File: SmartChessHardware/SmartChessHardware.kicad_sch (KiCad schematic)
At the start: 28 parts, among them IC1 Pi-Zero-UART, IC2 Arduino_UNO_R3, IC3 MCP23017x-x-SO, J1 Barrel_Jack

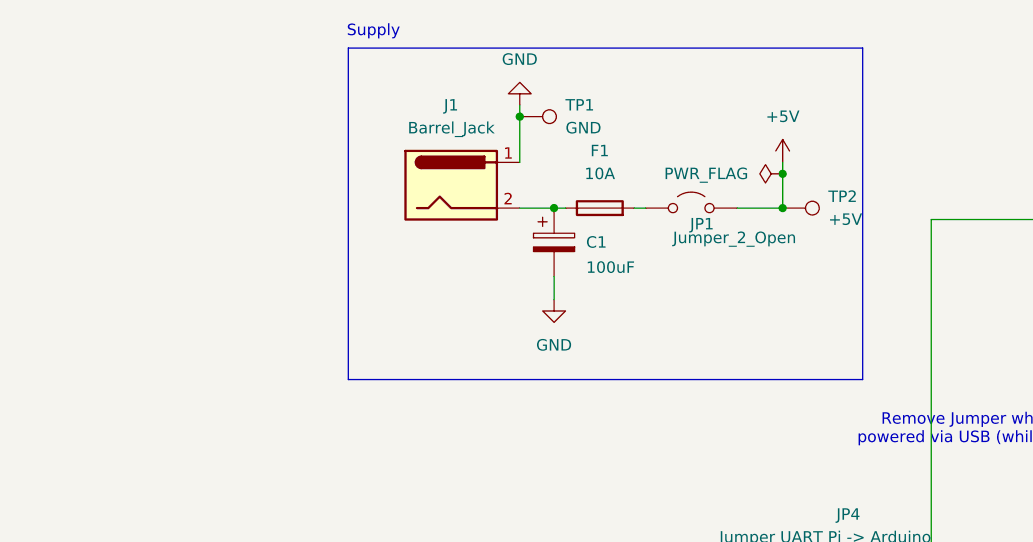
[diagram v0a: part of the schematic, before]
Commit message: Reworked supply circuit
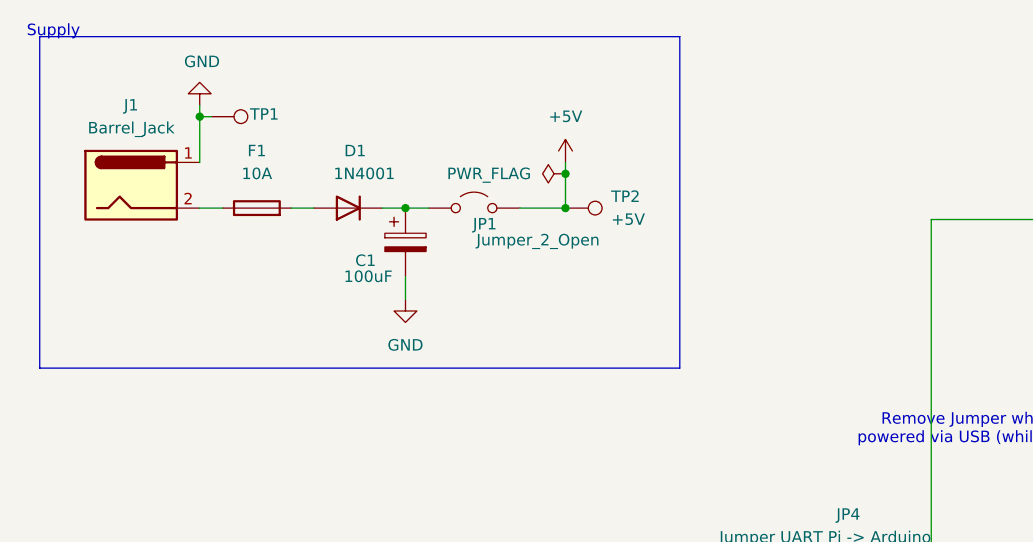
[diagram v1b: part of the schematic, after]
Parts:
- added D1: 1N4001, Diode_THT:D_DO-41_SOD81_P10.16mm_Horizontal, symbol Diode:1N4001
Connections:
- net at F1.1, J1.2: no longer C1.1
- net at JP1.1 (A): now also C1.1, D1.1 (K); no longer F1.2
- new net: D1.2 (A), F1.2
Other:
- moved on the sheet: C1, J1, JP1, TP1, TP2
